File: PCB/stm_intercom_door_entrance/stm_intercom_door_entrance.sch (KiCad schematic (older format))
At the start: 59 parts, among them J1 Screw_Terminal_01x02, J10 Conn_01x02, J11 Conn_01x04, J12 Conn_01x04, J13 Conn_01x04, J14 Screw_Terminal_01x02, J15 Conn_01x02, J16 Conn_01x01, J17 Screw_Terminal_01x03, J18 Screw_Terminal_01x03, J19 Conn_01x03, J2 Conn_01x04, J20 Conn_01x08, J23 Conn_01x02, J24 Conn_01x02, J3 Conn_01x04, J4 Conn_01x02, J5 Conn_01x04, J6 Conn_01x02, J7 Screw_Terminal_01x02, J8 Conn_01x04, J9 Conn_01x04, K1 SANYOU_SRD_Form_C, K2 SANYOU_SRD_Form_C, Q1 2N2219, Q2 2N2219, U1 YAAJ_BluePill_Part_Like, U2 MCP2551-I-P, U3 MAX3232_convertor, U4 4N25, U5 L7805, U6 4N25

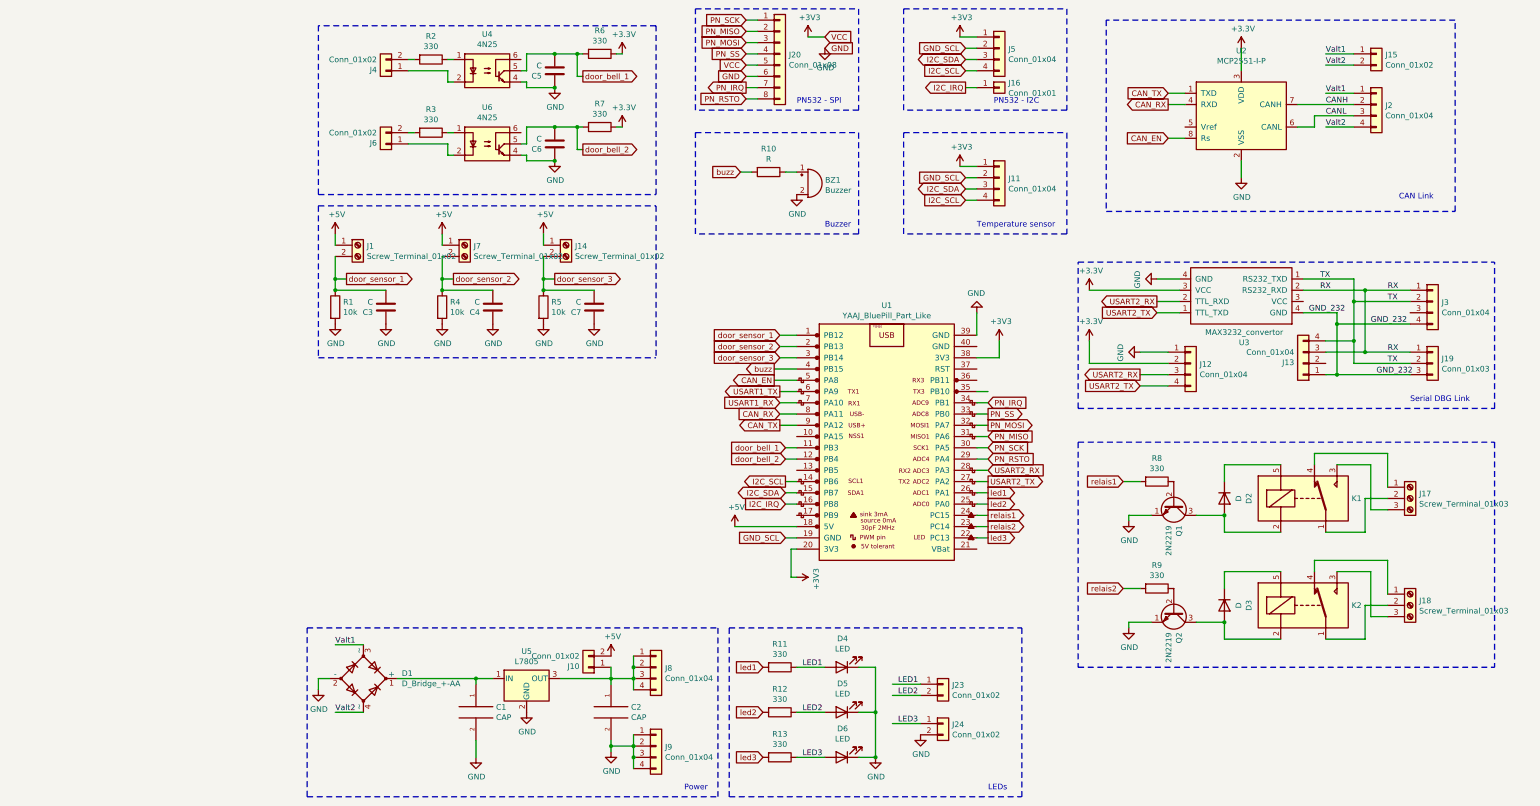
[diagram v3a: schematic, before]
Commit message: update PCB
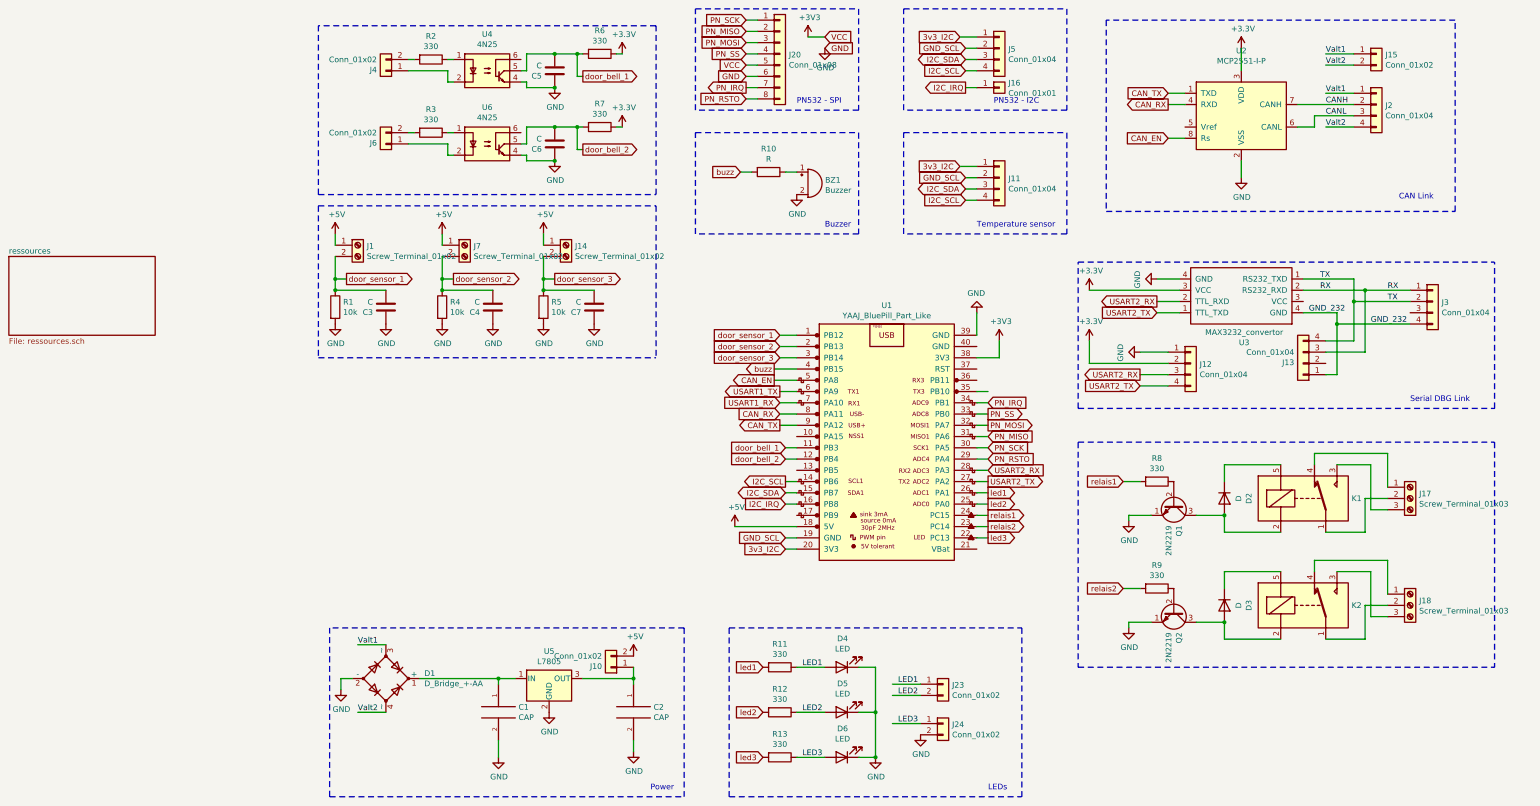
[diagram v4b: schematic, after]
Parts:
- removed J19: Conn_01x03, Connector_PinHeader_2.54mm:PinHeader_1x03_P2.54mm_Vertical, symbol Connector_Generic:Conn_01x03
- removed J8, J9: Conn_01x04, Connector_PinHeader_2.54mm:PinHeader_1x04_P2.54mm_Vertical, symbol Connector_Generic:Conn_01x04
- R10: footprint Resistor_THT:R_Axial_DIN0204_L3.6mm_D1.6mm_P2.54mm_Vertical -> Resistor_THT:R_Axial_DIN0207_L6.3mm_D2.5mm_P10.16mm_Horizontal
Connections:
- net +3V3: no longer J11.1 (Pin_1), J5.1 (Pin_1), U1.20 (3V3)
- new net 3v3_I2C: J11.1 (Pin_1), J5.1 (Pin_1), U1.20 (3V3)
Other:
- moved on the sheet: C1, C2, D1, J10, U5
